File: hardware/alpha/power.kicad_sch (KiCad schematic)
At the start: 47 parts, among them J1 EXT POWER, J10 HOLE, J11 HOLE, J12 HOLE, J13 HOLE, J14 HOLE, J15 HOLE, P20 P20, P28 P28, Q3 IRLML2244, U11 TPS63700DRCT, U12 L79L05_SO8, U2 TPS61170DRVR, U6 TLE2082, U8 L78L05_SO8

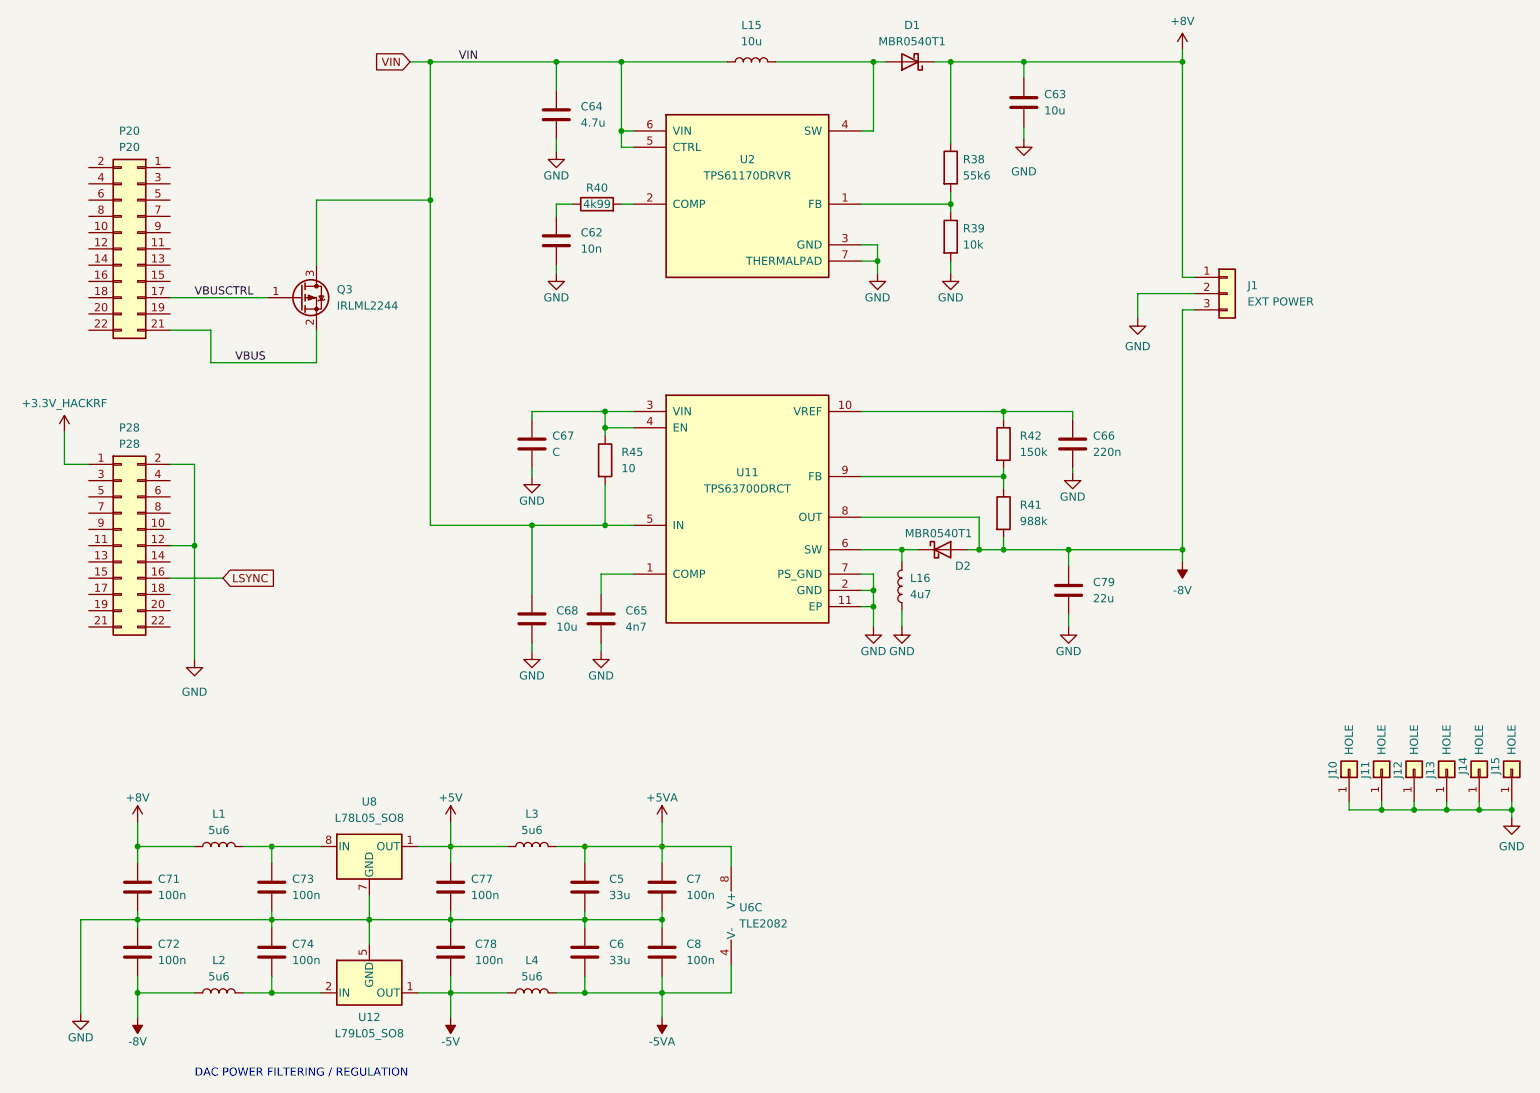
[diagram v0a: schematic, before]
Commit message: BOM WIP
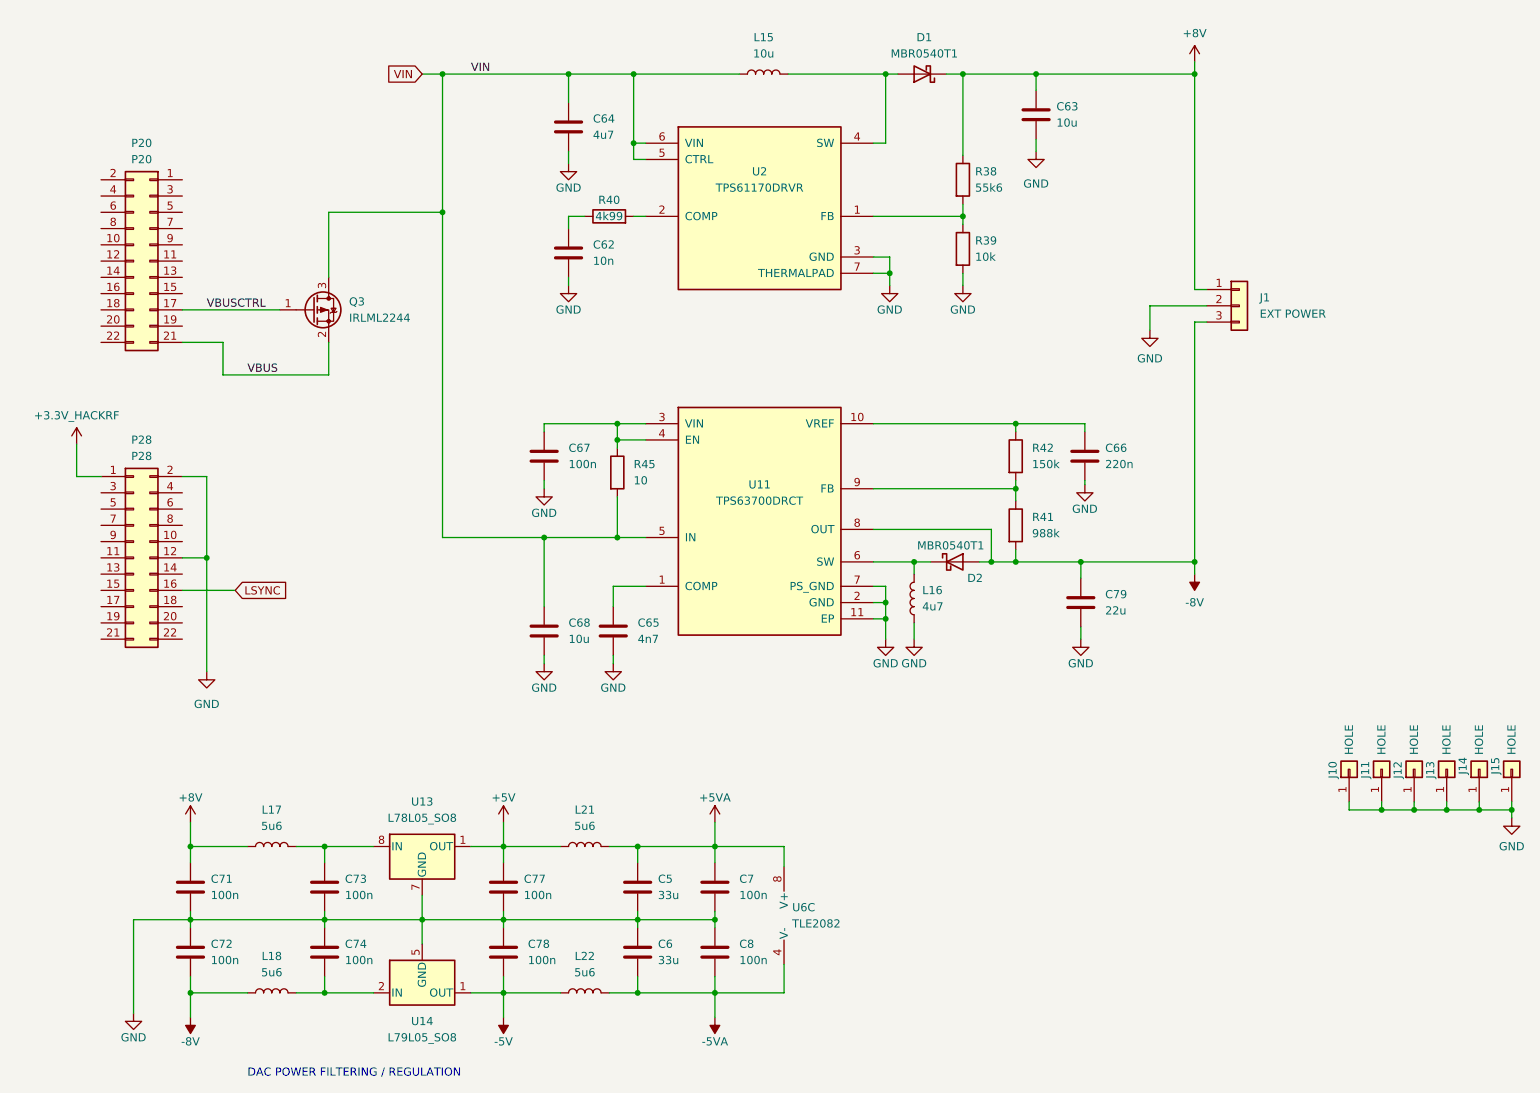
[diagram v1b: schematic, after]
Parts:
- C64: value 4.7u -> 4u7
- C67: value C -> 100n
- renumbered L1 to L17, L2 to L18, L3 to L21, L4 to L22, U8 to U13, U12 to U14
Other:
- moved on the sheet: C5, C6, C62, C63, C64, C65, C66, C67, C68, C7, C71, C72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
